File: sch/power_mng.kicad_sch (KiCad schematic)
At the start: 28 parts, among them J1 USB_C_Receptacle_USB2.0_16P, J3 Batt-Con, U2 TPS63061, U3 USBLC6-2P6, U5 TLV75801PDRV, U6 TLV75533PDRV

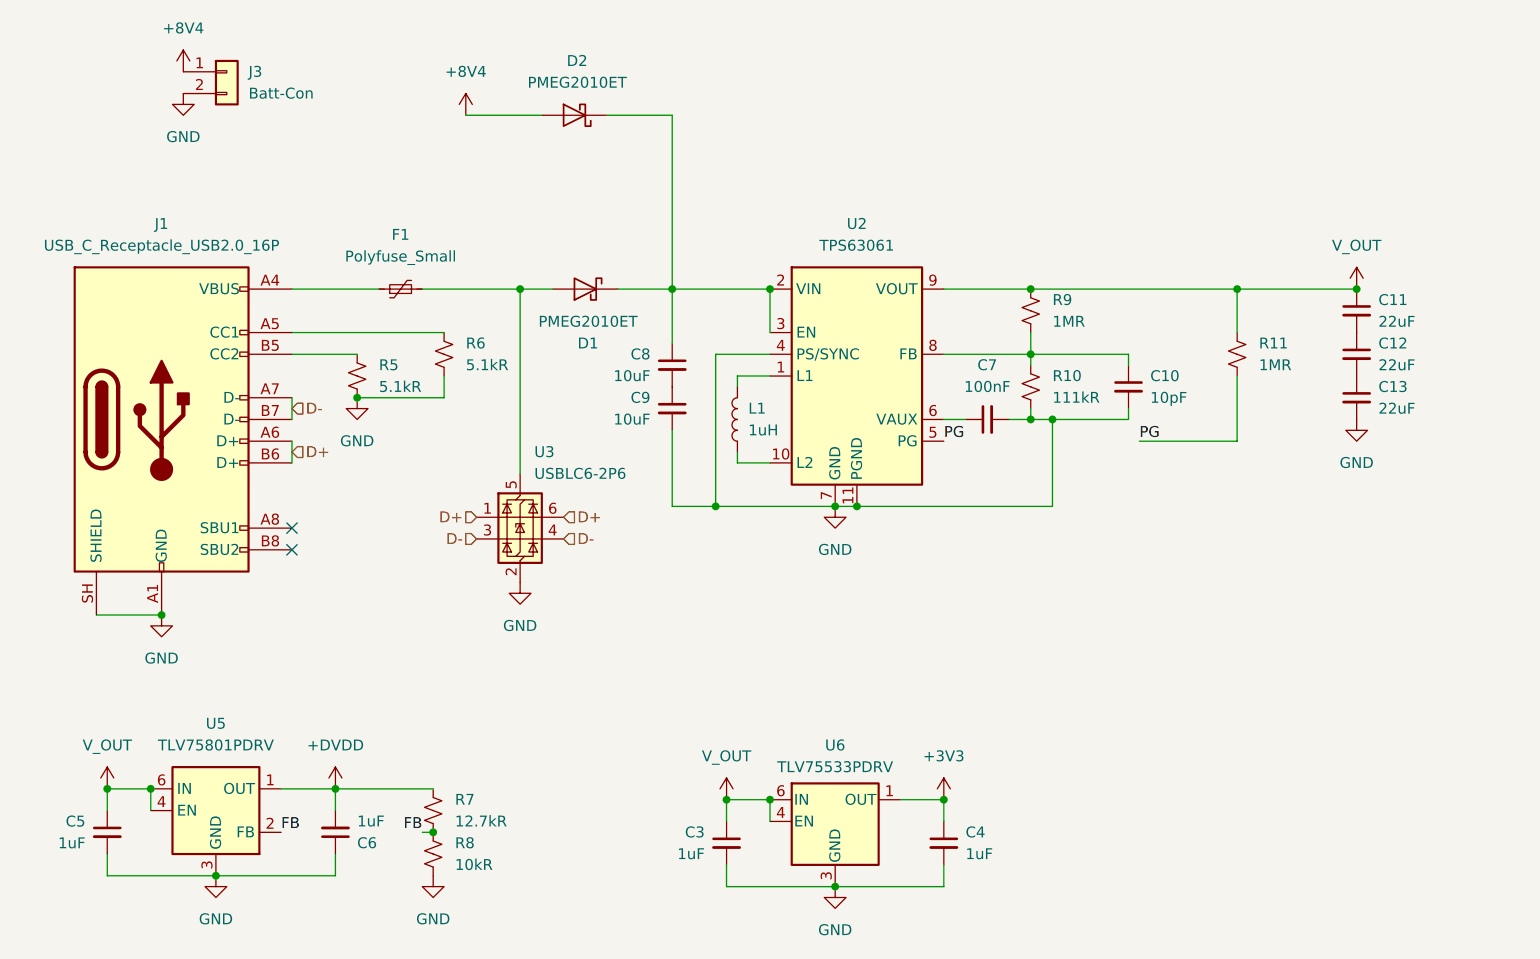
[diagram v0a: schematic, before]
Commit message: gah
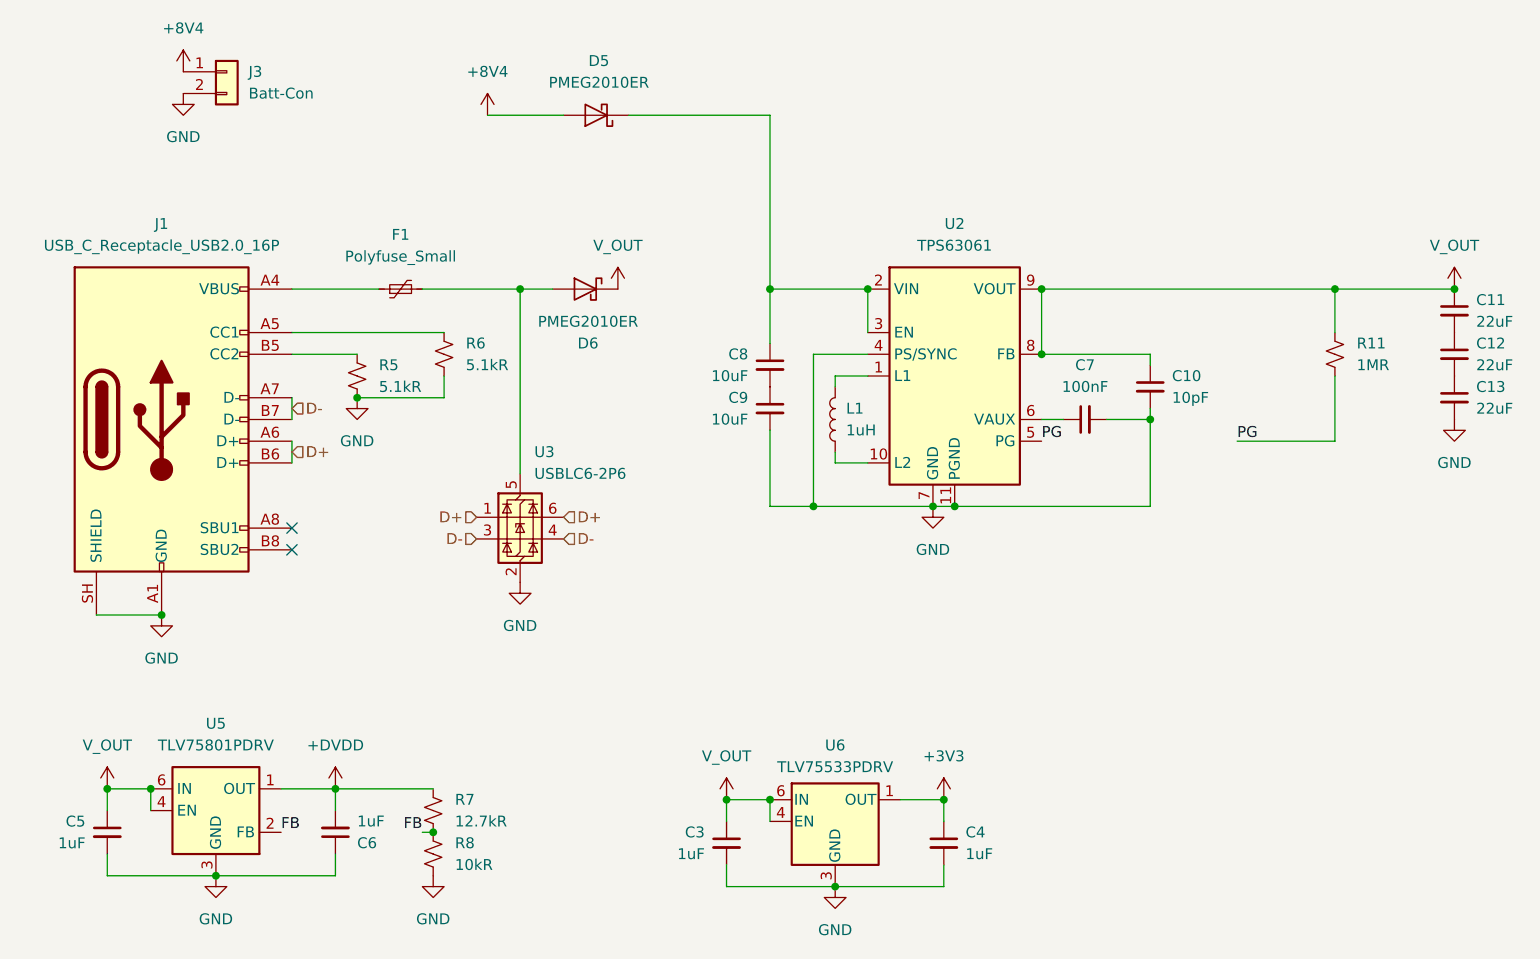
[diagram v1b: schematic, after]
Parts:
- removed D1, D2: PMEG2010ET, Package_TO_SOT_SMD:SOT-23, symbol Diode:PMEG2010ET
- removed R10: 111kR, Resistor_SMD:R_0402_1005Metric, symbol Device:R_Small_US
- removed R9: 1MR, Resistor_SMD:R_0402_1005Metric, symbol Device:R_Small_US
- added D5, D6: PMEG2010ER, Diode_SMD:Nexperia_CFP3_SOD-123W, symbol Diode:PMEG2010ER
- C3, C4, C5, C6: footprint Capacitor_SMD:C_0201_0603Metric -> Capacitor_SMD:C_01005_0402Metric
- F1: footprint Fuse:Fuse_0402_1005Metric -> Fuse:Fuse_0603_1608Metric
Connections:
- net +8V4: now also D5.2 (A)
- net V_OUT: now also C10.1, U2.8 (FB), D6.1 (K)
- net at F1.2, U3.5 (VBUS): now also D6.2 (A)
- net at C8.1, U2.2 (VIN), U2.3 (EN): now also D5.1 (K)
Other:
- moved on the sheet: C10, C11, C12, C13, C7, C8, C9, L1, R11, U2
